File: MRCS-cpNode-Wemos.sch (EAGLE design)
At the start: 40 parts, among them CON1 3.5MM, CON2 3.5MM, J2 CONNECTOR-GROVE-4P-2.0-347013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, Q2 2n7002, Q3 2n7002, Q4 2n7002, Q5 2n7002, U3 NE555P, U4 MAX3465CPD

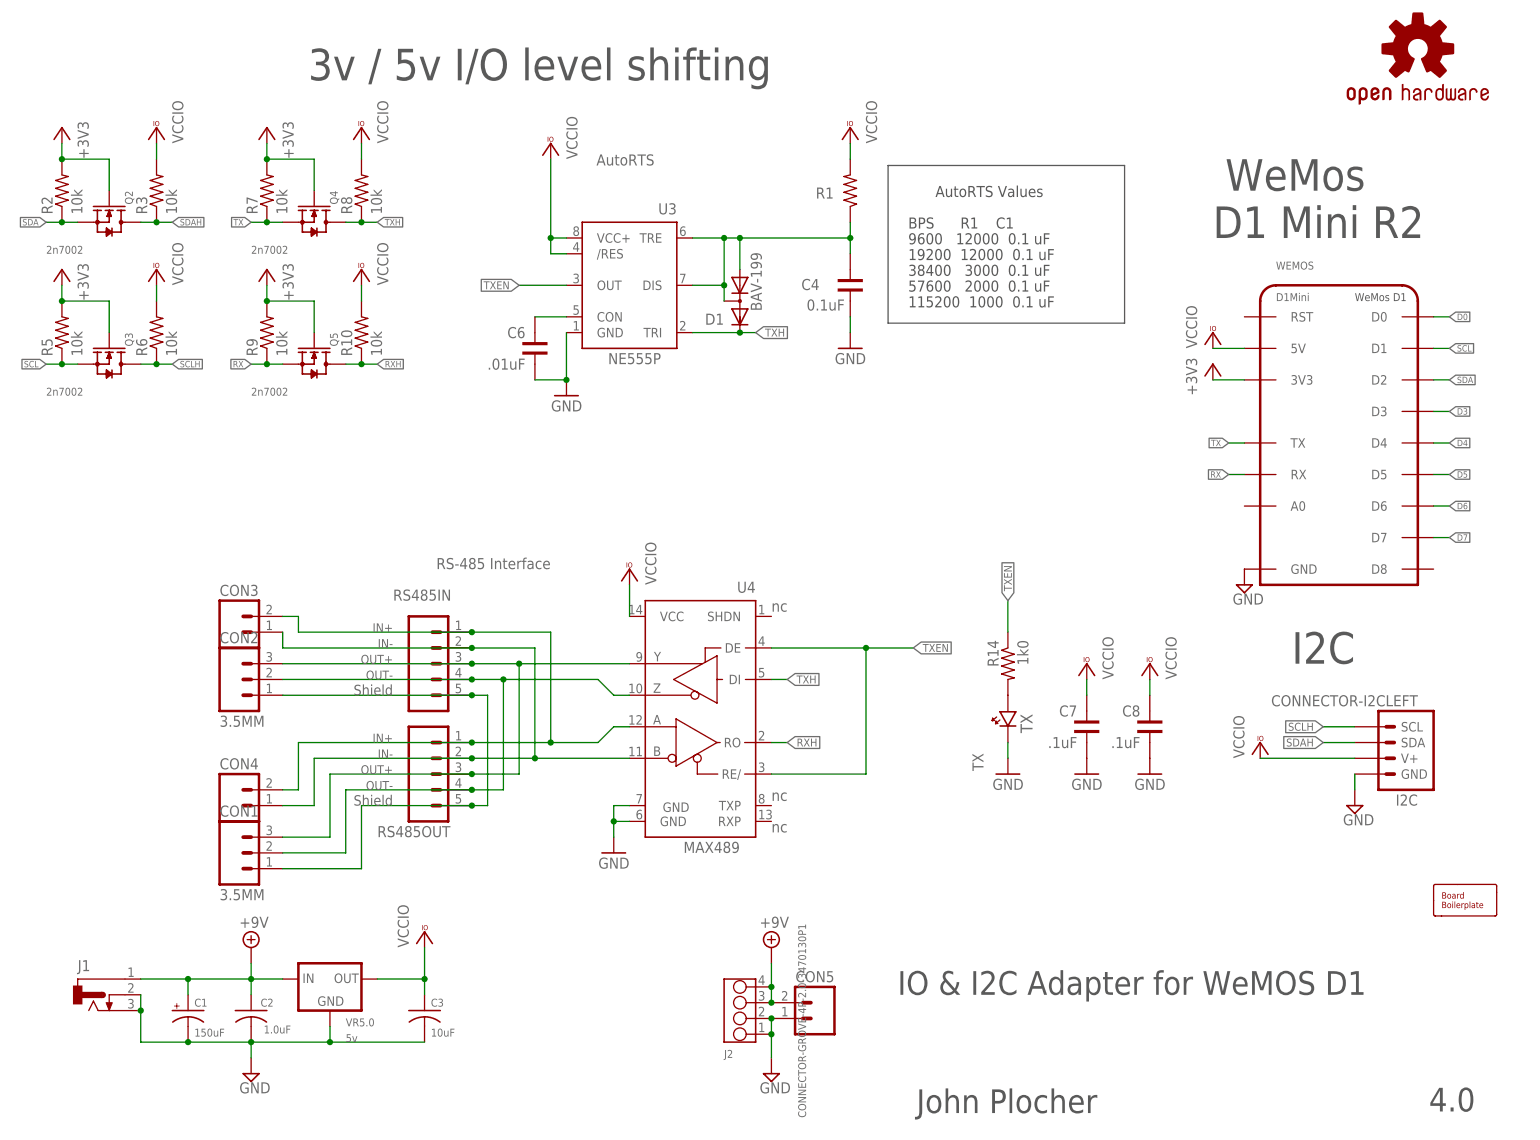
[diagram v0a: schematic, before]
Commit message: 5.0
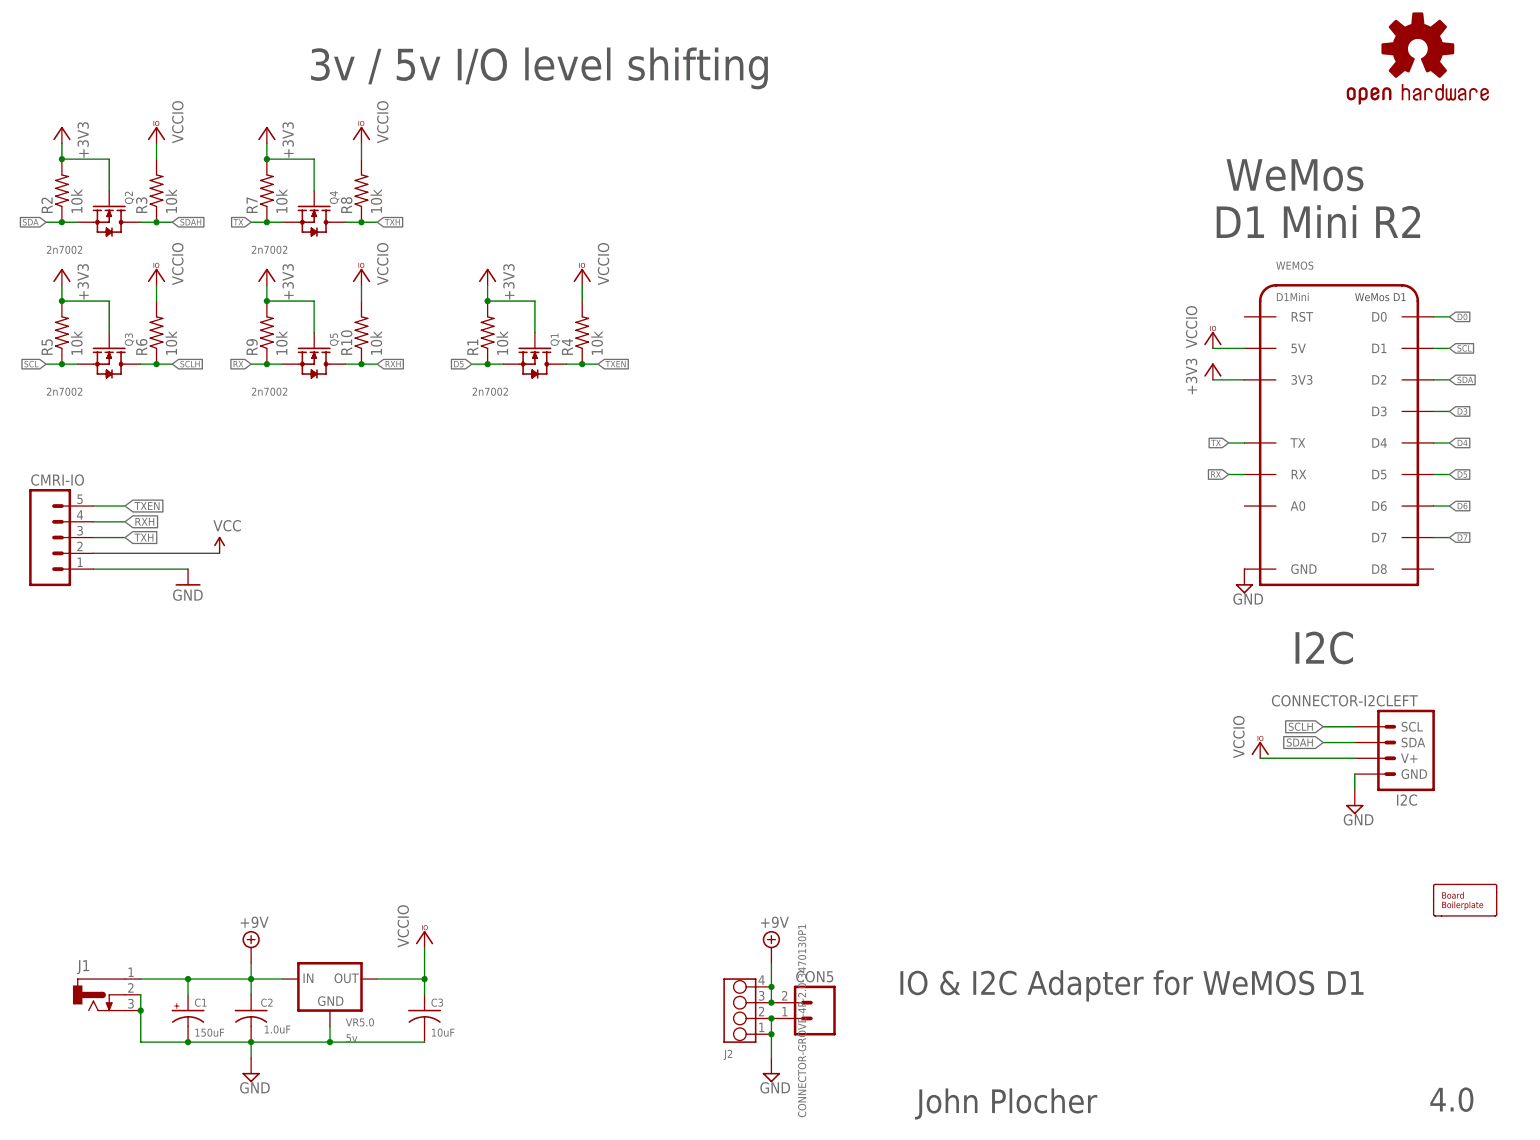
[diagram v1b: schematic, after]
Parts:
- removed C4: 0.1uF, SPCoast:CC0805
- removed C6: .01uF, SPCoast:CC0805
- removed C7: .1uF, SPCoast:CC0805
- removed C8: .1uF, SPCoast:CC0603
- removed CON1, CON2: 3.5MM, SPCoast:CONNECTOR-M035MM-LOCK
- removed CON3, CON4: (no value), SPCoast:CONNECTOR-M025MM-LOCK
- removed D1: BAV-199, SPCoast:DIODE-BAV199
- removed R14: 1k0, SPCoast:R0805-RES
- removed RS485IN: (no value), SparkFun:M05PTH
- removed RS485OUT: (no value), SparkFun:M05LOCK
- removed TX: TX, SPCoast:LED0603-LED
- removed U3: NE555P, SparkFun:NE555P
- removed U4: MAX3465CPD, maxim:MAX3465CPD
- added CMRI-IO: (no value), SPCoast:CONNECTOR-M05LOCK_LONGPADS
- added Q1: 2n7002, SPCoast:MOSFET-N-BSS138-SOT23
- added R4: 10k, SPCoast:R0805-RES
- BOARD: device SPCoast:BOARD69X100 -> SPCoast:BOARD69X90
- R1: value (none) -> 10k; device SPCoast:RPTH-1/6W -> SPCoast:R0805-RES
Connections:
- removed net IN+: CON3.B, CON4.B, RS485IN.1, RS485OUT.1, U4.A
- removed net IN-: CON3.A, CON4.A, RS485IN.2, RS485OUT.2, U4.B
- removed net N$1: C4.1, D1.A, D1.AC, R1.1, U3.DIS, U3.TRE
- removed net N$29: R14.2, TX.A
- removed net N$38: C6.1, U3.CON
- removed net OUT+: CON1.3, CON2.3, RS485IN.3, RS485OUT.3, U4.Y
- removed net OUT-: CON1.2, CON2.2, RS485IN.4, RS485OUT.4, U4.Z
- removed net SHIELD: CON1.1, CON2.1, RS485IN.5, RS485OUT.5
- new net VCC: CMRI-IO.2
- net +3V3: now also Q1.G, R1.2
- net D5: now also Q1.S, R1.1
- net GND: now also CMRI-IO.1; no longer C4.2, C6.2, C7.2, C8.2, TX.C, U3.GND, U4.GND, U4.GND@1
- net RXH: now also CMRI-IO.4; no longer U4.RO
- net TXEN: now also CMRI-IO.5, Q1.D, R4.1; no longer R14.1, U3.OUT, U4.DE, U4.RE/
- net TXH: now also CMRI-IO.3; no longer D1.C, U3.TRI, U4.DI
- net VCCIO: now also R4.2; no longer C7.1, C8.1, R1.2, U3./RES, U3.VCC+, U4.VCC
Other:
- note removed: "115200 1000 0.1 uF"
- note removed: "19200 12000 0.1 uF"
- note removed: "38400 3000 0.1 uF"
- note removed: "57600 2000 0.1 uF"
- note removed: "9600 12000 0.1 uF"
- note removed: "AutoRTS"
- note removed: "AutoRTS Values"
- note removed: "BPS R1 C1"
- note removed: "IN+"
- note removed: "IN-"
- note removed: "MAX489"
- note removed: "OUT+"
- note removed: "OUT-"
- note removed: "RS-485 Interface"
- note removed: "Shield"
- note removed: "nc"
- moved on the sheet: R1
